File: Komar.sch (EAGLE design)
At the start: 112 parts, among them CON1 USB-VERTICAL, CON10 PINHEAD_1X01-2, CON11 PINHEAD_1X01-2, CON12 PINHEAD_1X01-2, CON13 PINHEAD_1X01-2, CON14 PINHEAD_1X01-2, CON15 PINHEAD_1X01-2, CON2 PINHEAD_1X01-2, CON3 CON-4P-TABS-STRAIGHT, CON4 CON-4P-TABS-STRAIGHT, CON5 CON-4P-TABS-STRAIGHT, CON6 CON-4P-TABS-STRAIGHT, CON7 CON-4P-TABS-STRAIGHT, CON8 PINHEAD_1X04-2, CON9 PINHEAD_1X01-2, IC1 TPD3S014DBVR-SOT23-6, IC2 TPD3S014DBVR-SOT23-6, IC3 ATA6561-GBQW-N-HVSON8, IC4 ATA6561-GBQW-N-HVSON8, IC5 MCP9700AT-E/TTVAO-SOT23, IC6 11LC040T-E/TT, Q1 FDMS86368-F085, Q10 FDMS86368-F085, Q11 FDMS86368-F085, Q12 FDMS86368-F085, Q2 FDMS86368-F085, Q3 FDMS86368-F085, Q4 FDMS86368-F085, Q5 FDMS86368-F085, Q6 FDMS86368-F085, Q7 FDMS86368-F085, Q8 FDMS86368-F085, Q9 FDMS86368-F085

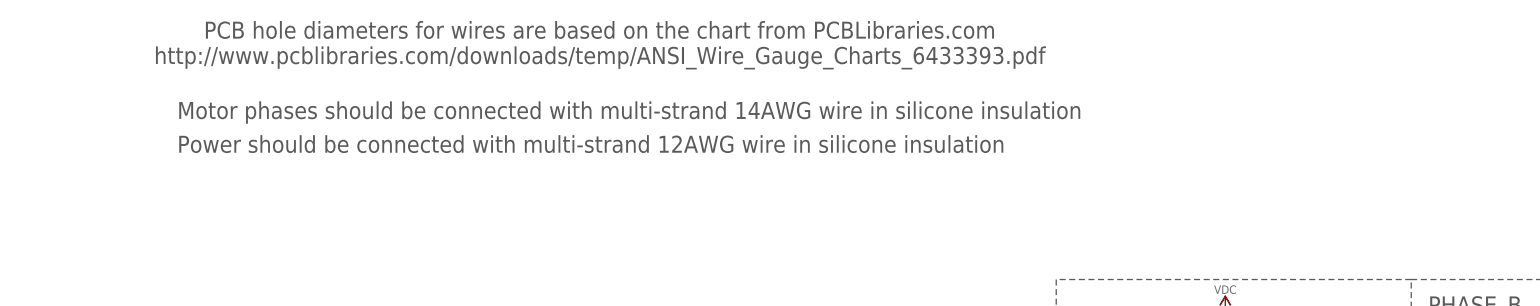
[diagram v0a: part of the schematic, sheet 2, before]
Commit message: manufacturing instruction update
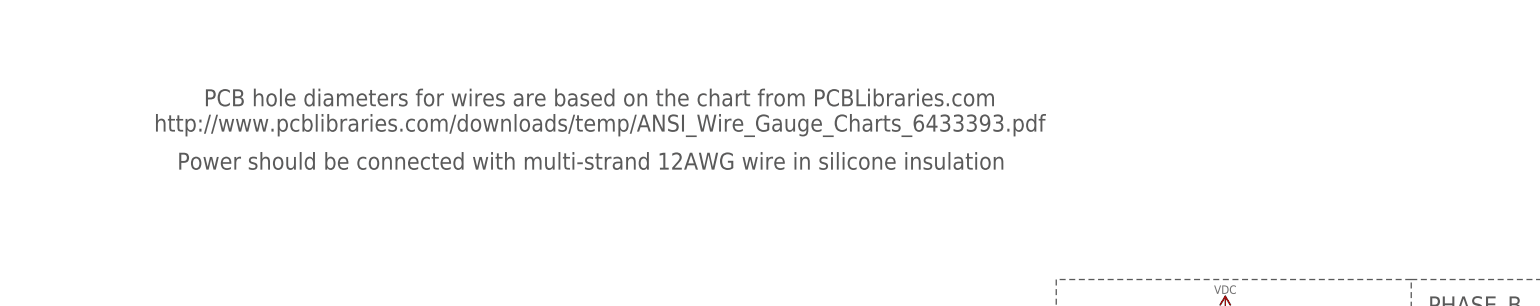
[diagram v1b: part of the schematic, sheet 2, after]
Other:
- note removed: "Motor phases should be connected with multi-strand 14AWG wire in silicone insulation"
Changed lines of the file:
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@@
 <wire x1="233.68" y1="30.48" x2="233.68" y2="73.66" width="0.1524" layer="97" style="shortdash"/>
 <wire x1="233.68" y1="73.66" x2="180.34" y2="73.66" width="0.1524" layer="97" style="shortdash"/>
-<text x="5.08" y="276.86" size="2.54" layer="97" font="vector" ratio="15" align="center-left">Motor phases should be connected with multi-strand 14AWG wire in silicone insulation</text>
-<text x="5.08" y="271.78" size="2.54" layer="97" font="vector" ratio="15" align="center-left">Power should be connected with multi-strand 12AWG wire in silicone insulation</text>
-<text x="68.58" y="287.02" size="2.54" layer="97" font="vector" ratio="15" align="center">PCB hole diameters for wires are based on the chart from PCBLibraries.com
+<text x="5.08" y="269.24" size="2.54" layer="97" font="vector" ratio="15" align="center-left">Power should be connected with multi-strand 12AWG wire in silicone insulation</text>
+<text x="68.58" y="276.86" size="2.54" layer="97" font="vector" ratio="15" align="center">PCB hole diameters for wires are based on the chart from PCBLibraries.com
 http://www.pcblibraries.com/downloads/temp/ANSI_Wire_Gauge_Charts_6433393.pdf</text>
 </plain>
